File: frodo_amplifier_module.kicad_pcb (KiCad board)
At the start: 4 copper layers, 24.5 x 12.5 mm, 37 parts, among them IC1 INA826AID, J1 JST-GH, J2 JST-GH, J3 JST-GH, J4 JST-GH, U1 ADC101C021CIMK, U2 MCP6001-OT, U3 MIC5504-3.3YM5, U4 REF3033

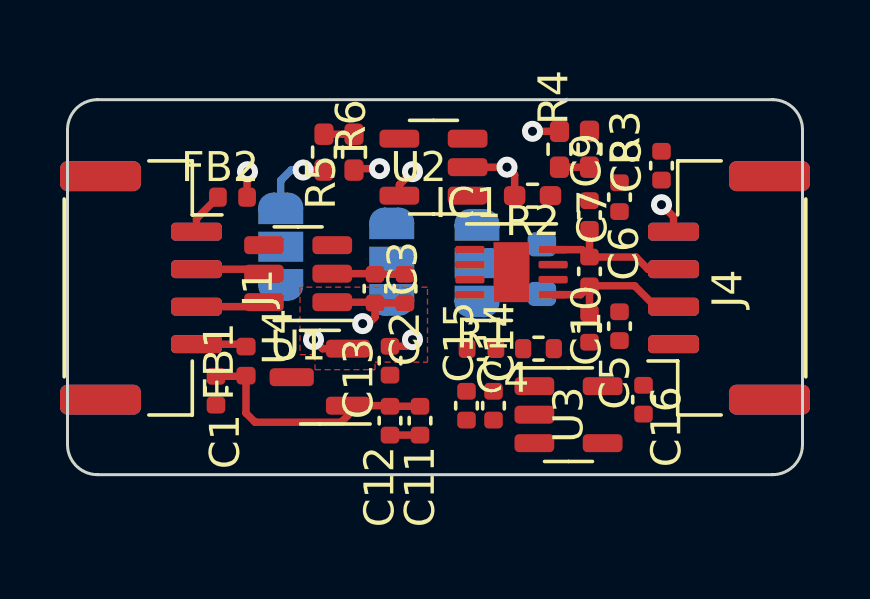
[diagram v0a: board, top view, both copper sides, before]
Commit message: finished routing -> pcb should be ready to order after review
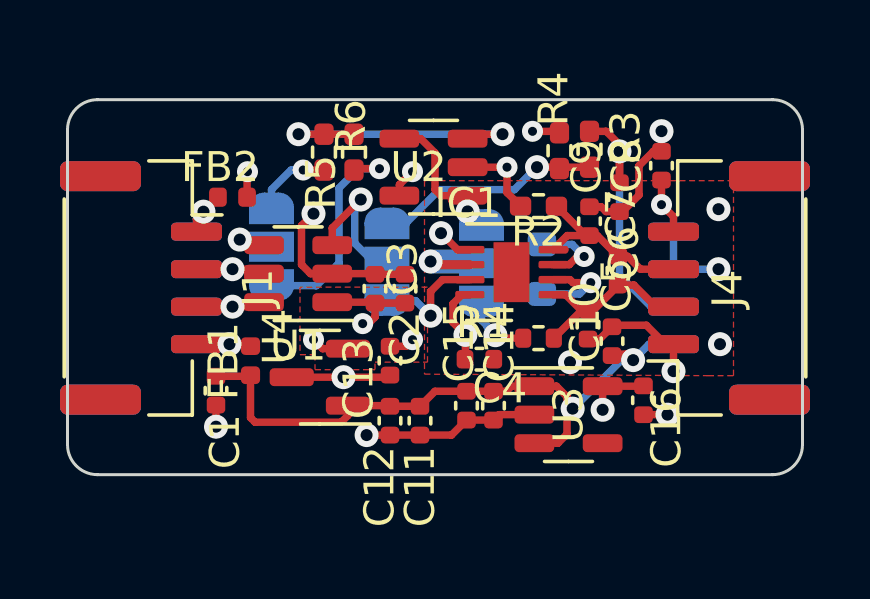
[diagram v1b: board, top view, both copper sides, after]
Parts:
- moved C7 0.95 mm to (69.3, 39.7)
- moved C5 0.56 mm to (69.2, 42.0), turned to 90 degrees
- moved R2 0.40 mm to (66.7, 37.5)
- moved C4 0.36 mm to (64.7, 42.6)
- moved R1 0.35 mm to (66.7, 42.0)
- moved JP2 0.31 mm to (57.8, 38.9)
- moved C9 0.20 mm to (68.4, 38.0)
- moved JP1 0.16 mm to (61.6, 39.4)
- moved FB1 0.15 mm to (57.1, 42.7)
- moved JP3 0.15 mm to (64.8, 39.5)
- moved C10 0.12 mm to (68.3, 41.5)
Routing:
- net GND: track 10.1 -> 38.6 mm, vias 4 -> 17
- net 5V: track 8.61 -> 22.5 mm, vias 0 -> 2
- net 3V3: track 2.92 -> 15.3 mm, vias 3 -> 5
- net Net-(J3-Pin_3): track 0.00 -> 9.86 mm, vias 0 -> 1
- net Net-(U2-+): track 1.00 -> 9.88 mm, vias 0 -> 2
- net sig2: track 1.00 -> 7.52 mm, vias 0 -> 1
- net Net-(JP1-C): track 0.00 -> 4.94 mm, vias 0 -> 1
- net Net-(JP3-B): track 0.00 -> 4.86 mm, vias 0 -> 1
- net sig: track 0.00 -> 3.94 mm, vias 0 -> 1
- net Net-(IC1-RG_1): track 0.00 -> 3.08 mm, vias 0 -> 1
- net ref: track 0.00 -> 2.93 mm, vias 0 -> 1
- net Net-(IC1-RG_2): track 0.00 -> 2.72 mm, vias 0 -> 1
- net Net-(JP2-C): track 0.00 -> 2.04 mm, vias 0 -> 1
- net Net-(J1-Pin_4): track 1.68 -> 3.08 mm, vias 0 -> 1
- net +IN: track 5.33 -> 6.58 mm
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- added copper zone on F.Cu, net GND
